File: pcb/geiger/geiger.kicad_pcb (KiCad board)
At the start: 2 copper layers, 160 x 112.4 mm, 105 parts, among them J1 Conn_01x02, J2 Conn_01x02, J3 Conn_01x03, J4 Conn_01x06, J5 Conn_01x02, J6 Conn_02x05_Odd_Even, J7 Conn_02x05_Odd_Even, K1 RELAY_DPST, K2 RELAY_DPST, Q1 BC107, Q2 BC140, Q3 BC160, Q4 IRF540N, Q5 BC140, Q6 BC140, Q7 BC307, Q8 BC847, Q9 BC847, U1 MSP430G2553_PW20, U2 74HC595, U3 AD558, U4 LM208, X1 5.7MHz

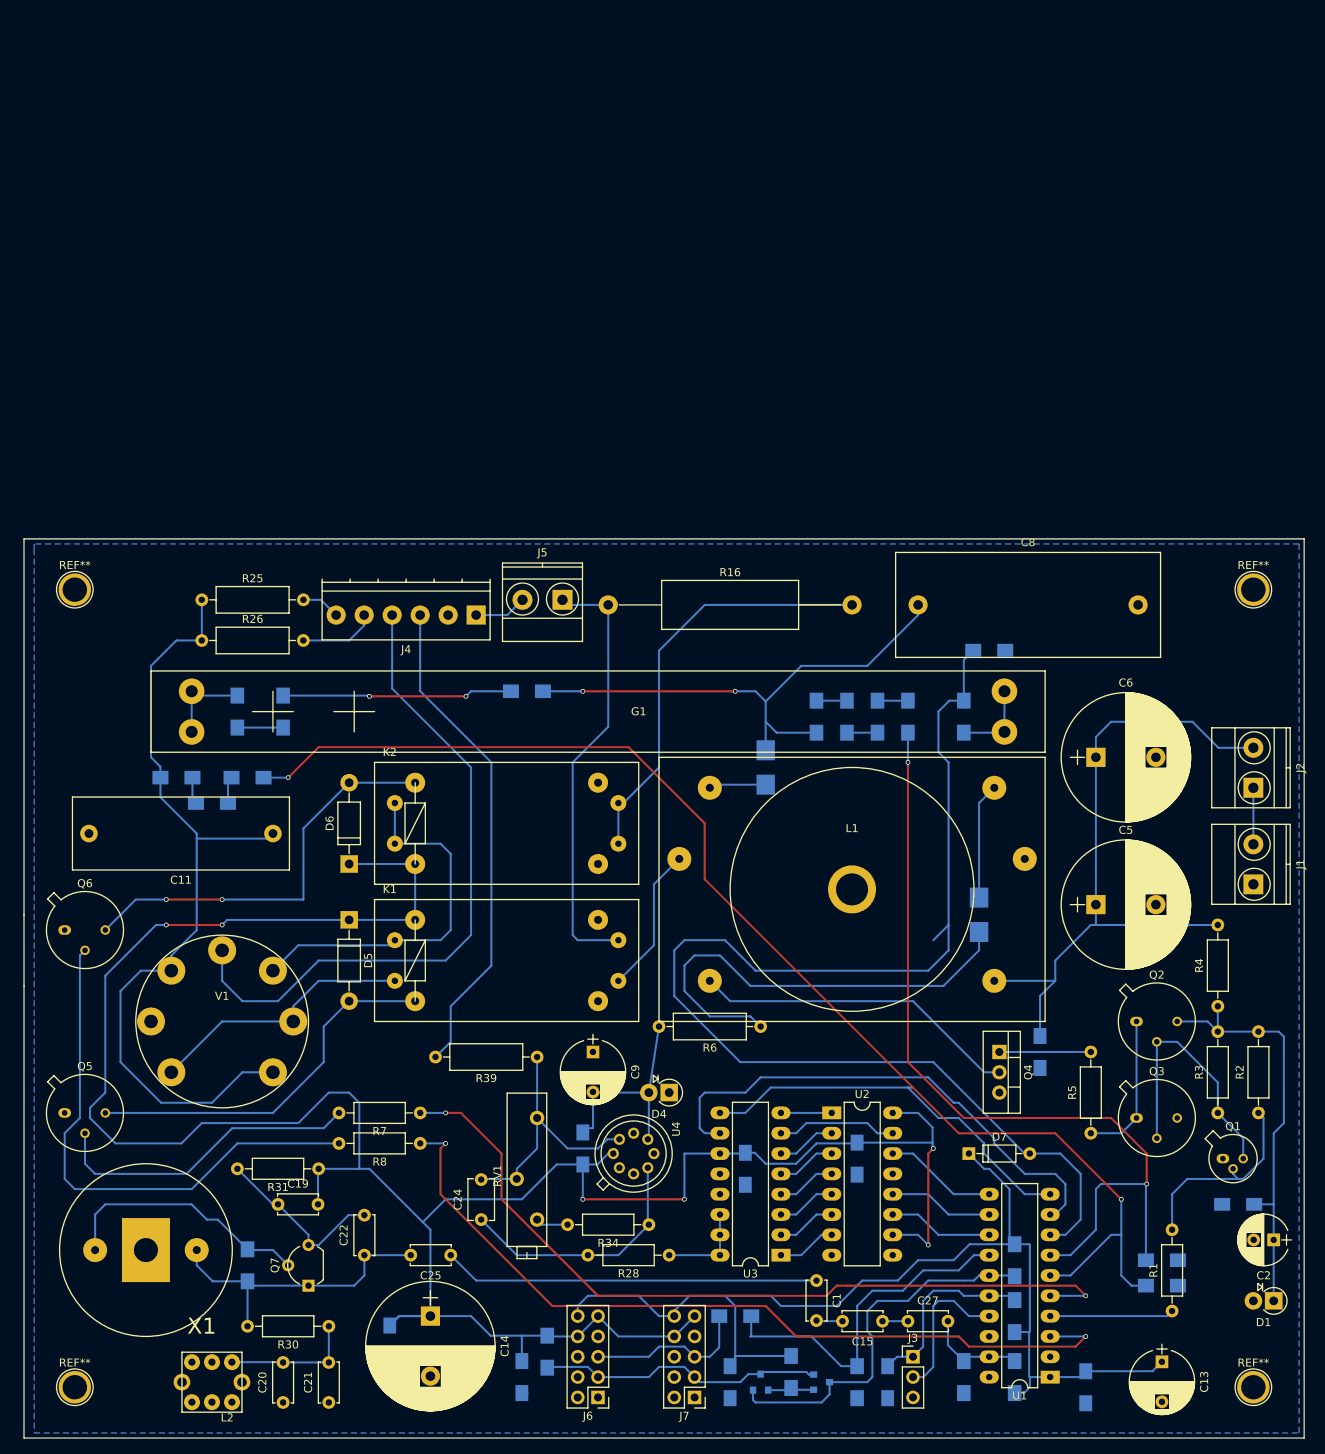
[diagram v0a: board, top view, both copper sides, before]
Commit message: Finish Geiger board.
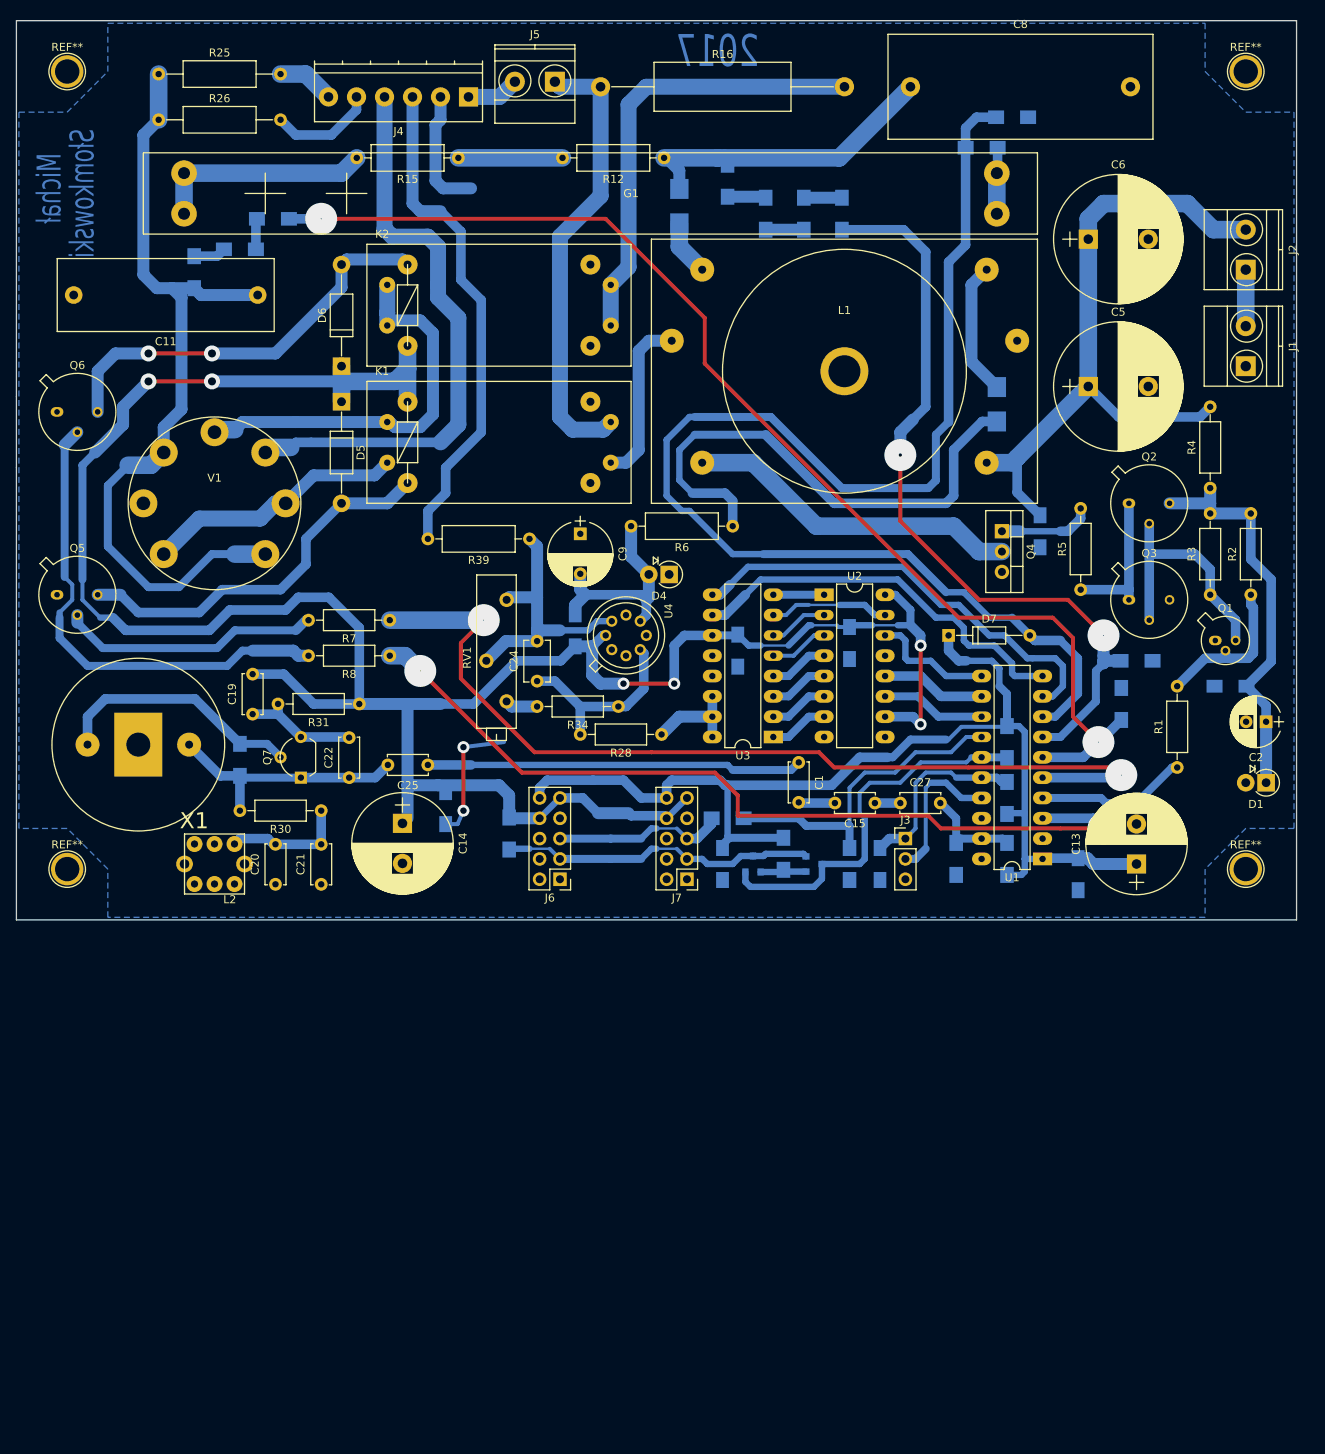
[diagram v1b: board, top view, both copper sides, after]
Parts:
- removed C17: 100n, Capacitors_SMD:C_1206_HandSoldering
- removed R17: 1M, Resistors_SMD:R_1206_HandSoldering
- C13: footprint Capacitors_ThroughHole:CP_Radial_D8.0mm_P5.00mm -> Capacitors_ThroughHole:CP_Radial_D12.5mm_P5.00mm
- C14: value 1000u -> 220u; footprint Capacitors_ThroughHole:CP_Radial_D16.0mm_P7.50mm -> Capacitors_ThroughHole:CP_Radial_D12.5mm_P5.00mm
- D5, D6: footprint Diodes_ThroughHole:D_DO-41_SOD81_P10.16mm_Horizontal -> Diodes_ThroughHole:D_DO-41_SOD81_P12.70mm_Horizontal
- D7: footprint Diodes_ThroughHole:D_DO-35_SOD27_P7.62mm_Horizontal -> Diodes_ThroughHole:D_DO-35_SOD27_P10.16mm_Horizontal
- R12: footprint Resistors_SMD:R_1206_HandSoldering -> Resistors_ThroughHole:R_Axial_DIN0309_L9.0mm_D3.2mm_P12.70mm_Horizontal; moved to F.Cu
- R15: value 1M -> 2M2; footprint Resistors_SMD:R_1206_HandSoldering -> Resistors_ThroughHole:R_Axial_DIN0309_L9.0mm_D3.2mm_P12.70mm_Horizontal; moved to F.Cu
- R25, R26: footprint Resistors_ThroughHole:R_Axial_DIN0309_L9.0mm_D3.2mm_P12.70mm_Horizontal -> Resistors_ThroughHole:R_Axial_DIN0309_L9.0mm_D3.2mm_P15.24mm_Horizontal
- moved R10 75.0 mm to (156.2, 95.9)
- moved R24 72.9 mm to (154.3, 101.3), turned to 90 degrees
- moved R15 72.6 mm to (71.4, 33.0), turned to 180 degrees
- moved R19 71.2 mm to (136.8, 31.8), turned to 180 degrees
- moved D3 71.0 mm to (99.1, 39.1)
- moved R23 69.9 mm to (48.3, 40.6)
- moved R22 69.3 mm to (44.1, 44.5)
- moved R12 68.8 mm to (97.2, 33.0)
- moved R5 68.0 mm to (149.2, 87.0)
- moved R1 67.9 mm to (161.3, 109.2)
- moved R9 67.9 mm to (105.1, 35.9), turned to 270 degrees
- moved C24 67.7 mm to (81.3, 98.4)
- moved C11 67.3 mm to (46.4, 50.2)
- moved C16 67.0 mm to (69.8, 114.3)
- moved R20 66.7 mm to (140.7, 27.9)
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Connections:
- R15 pad 2: Net-(R15-Pad2) -> Net-(G1-PadA)
- U1 pad 10: DAC_CE -> DAC_CS
- U1 pad 9: DAC_CS -> DAC_CE
- V1 pad 3: Net-(K1-Pad7) -> Net-(J4-Pad4)
- V1 pad 4: Net-(J4-Pad4) -> Net-(K1-Pad7)
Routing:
- net GND: track 0.88 -> 32.0 mm, vias 0 -> 2
- net Net-(C8-Pad1): track 66.2 -> 41.9 mm, vias 2 -> 0
- net Net-(G1-PadA): track 11.0 -> 28.2 mm
- net REL_HEATER_2: track 101.5 -> 118.2 mm
- net Net-(R12-Pad2): track 28.8 -> 13.0 mm, vias 2 -> 0
- net DAC_CS: track 64.3 -> 49.8 mm
- net Net-(J4-Pad4): track 83.5 -> 73.0 mm
- net GM_VOL: track 107.9 -> 98.0 mm
- net EYE_VOL: track 160.4 -> 150.8 mm
- net GM_PULSE: track 157.0 -> 165.8 mm
- net Net-(D2-Pad2): track 57.6 -> 66.3 mm
- net DAC_CE: track 49.5 -> 56.6 mm
- net Net-(C24-Pad1): track 31.5 -> 24.5 mm
- net Net-(C19-Pad1): track 22.1 -> 15.2 mm
- net Net-(Q5-Pad2): track 39.2 -> 32.6 mm
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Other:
- rule via_min_drill: 0.3 -> 0
- board text added: "2017"
- board text added: "Michał"
- board text added: "Słomkowski"
